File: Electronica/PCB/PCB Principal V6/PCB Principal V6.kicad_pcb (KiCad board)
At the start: 2 copper layers, 139.1 x 70 mm, 19 parts, among them J1 Conexion Sensores, J12 TP, J2 Power Monster, J3 On/Off General, J4 Power Input 2, J5 IDC Placa Botones, J6 Power Input 1, J7 Conn_01x01_Pin, J8 Conn_01x01_Pin, SW1 On/Off Motores

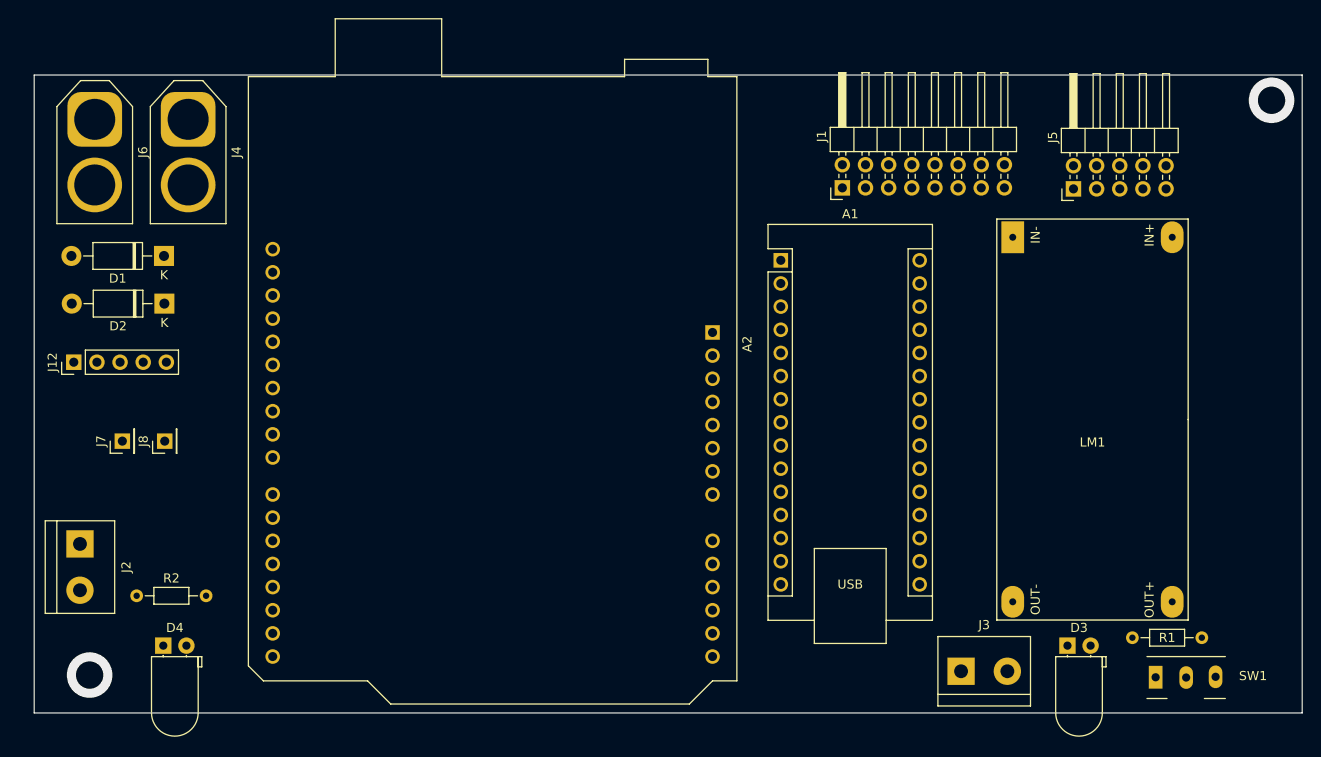
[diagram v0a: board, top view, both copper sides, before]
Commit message: pcb terminar?
TONTO EL QUE LEE
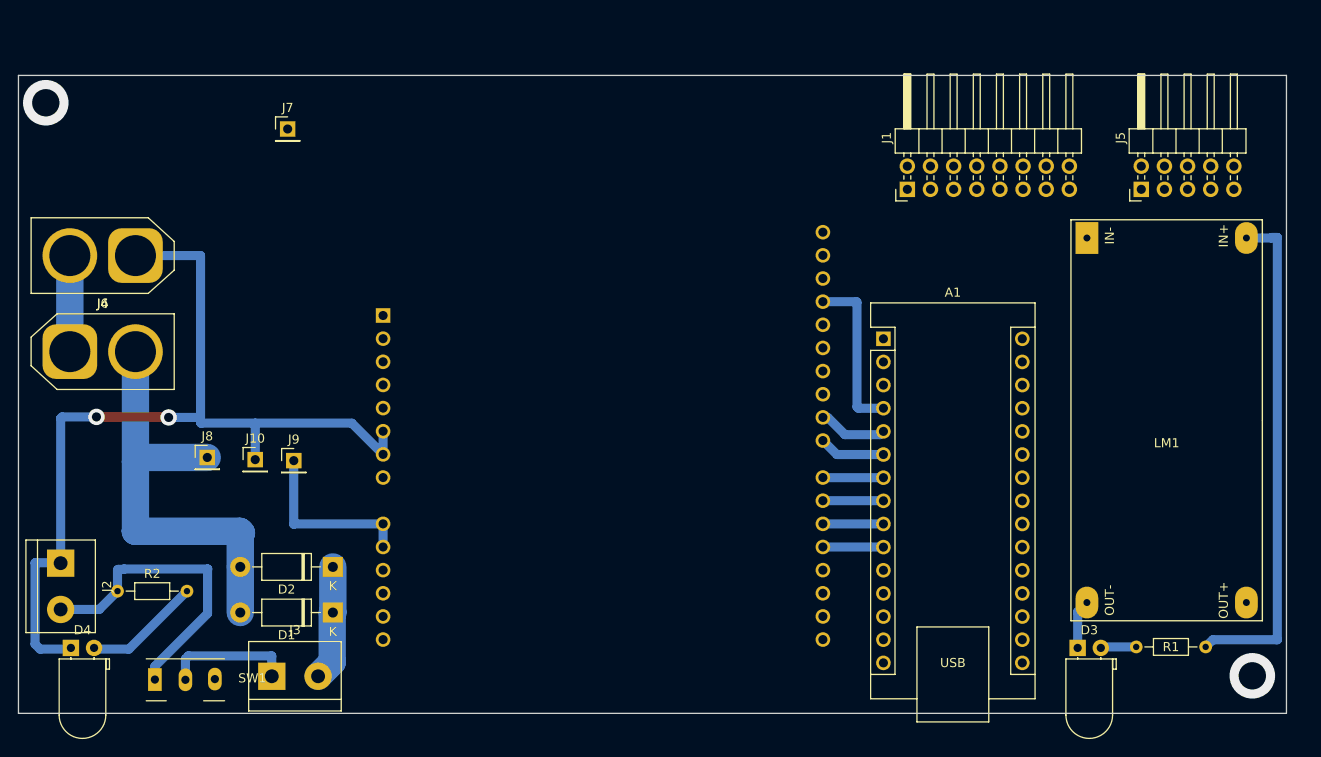
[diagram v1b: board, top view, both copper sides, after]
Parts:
- removed J12: TP, Connector_PinHeader_2.54mm:PinHeader_1x05_P2.54mm_Vertical
- added J10: Conn_01x01, Connector_PinHeader_2.54mm:PinHeader_1x01_P2.54mm_Vertical, F.Cu at (150.7, 67.6)
- added J9: Conn_01x01, Connector_PinHeader_2.54mm:PinHeader_1x01_P2.54mm_Vertical, F.Cu at (154.9, 67.7)
- A2: moved to B.Cu
- J7, J8: value Conn_01x01_Pin -> Conn_01x01
- moved SW1 109.8 mm to (141.0, 91.7)
- moved J3 75.6 mm to (152.5, 91.3)
- moved D1 43.3 mm to (159.2, 84.3)
- moved J7 38.8 mm to (154.2, 31.3), turned to 0 degrees
- moved A2 36.2 mm to (164.7, 51.7)
- moved D2 34.3 mm to (159.2, 79.3)
- moved J6 25.6 mm to (130.3, 55.7), turned to 0 degrees
- moved J4 16.0 mm to (137.5, 45.2), turned to 180 degrees
- moved A1 14.2 mm to (219.6, 54.3)
- moved D4 10.1 mm to (130.5, 88.2)
- moved LM1 8.14 mm to (250.7, 63.2)
- moved J5 7.44 mm to (247.9, 37.9)
- moved J1 7.13 mm to (222.2, 37.9)
- moved J8 5.00 mm to (145.4, 67.3), turned to 0 degrees
- moved J2 2.99 mm to (129.3, 78.9)
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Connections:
- J7 pad 1: +5V -> VNano
- J8 pad 1: GND -> PI+
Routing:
- net GND: track 0.00 -> 124.3 mm, vias 0 -> 2
- net MOTORES: track 0.00 -> 69.9 mm
- net PI+: track 0.00 -> 48.3 mm
- net Net-(J2-Pin_2): track 0.00 -> 33.9 mm
- net +5V: track 0.00 -> 19.3 mm
- net Net-(D4-A): track 0.00 -> 12.8 mm
- net Net-(D1-K): track 0.00 -> 12.7 mm
- net Net-(J4-Pin_2): track 0.00 -> 10.5 mm
- net BIN 2 MONSTER SHIELD: track 0.00 -> 7.57 mm
- net AIN2 MONSTER SHIELD: track 0.00 -> 7.28 mm
- net PWM B MONSTER SHIELD: track 0.00 -> 6.65 mm
- net PWM A MONSTER SHIELD: track 0.00 -> 6.65 mm
- net BIN 1 MONSTER SHIELD: track 0.00 -> 6.65 mm
- net AIN1 MONSTER SHIELD: track 0.00 -> 6.65 mm
- net Net-(D3-A): track 0.00 -> 3.93 mm
